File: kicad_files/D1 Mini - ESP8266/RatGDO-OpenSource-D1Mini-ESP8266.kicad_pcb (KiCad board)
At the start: 2 copper layers, 51.8 x 65.8 mm, 24 parts, among them J1 Screw_Terminal_01x03, J2 Conn_01x11, J3 Screw_Terminal_01x02, Q1 2N7002, Q2 AO3400A, Q3 AO3400A, Q4 AO3400A, U1 WeMos_D1_mini, U2 K7805-500R3

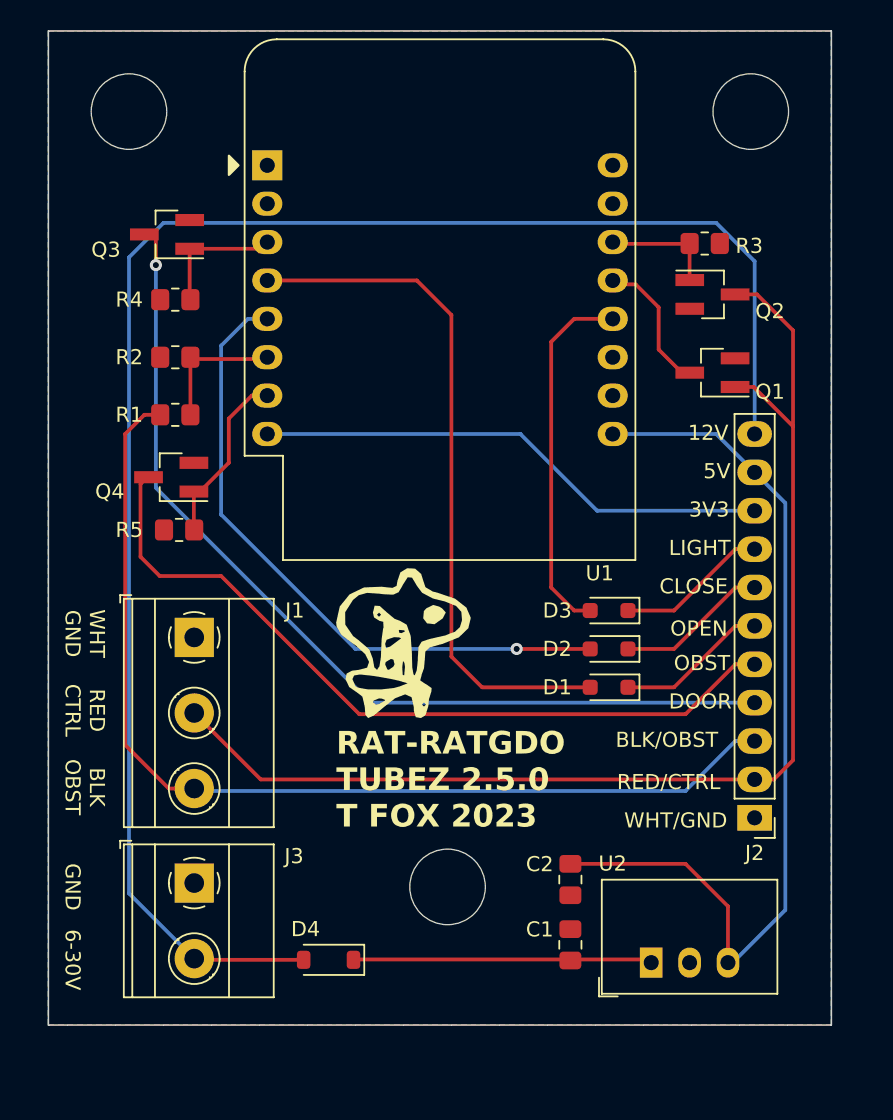
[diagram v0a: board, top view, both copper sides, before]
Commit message: rename
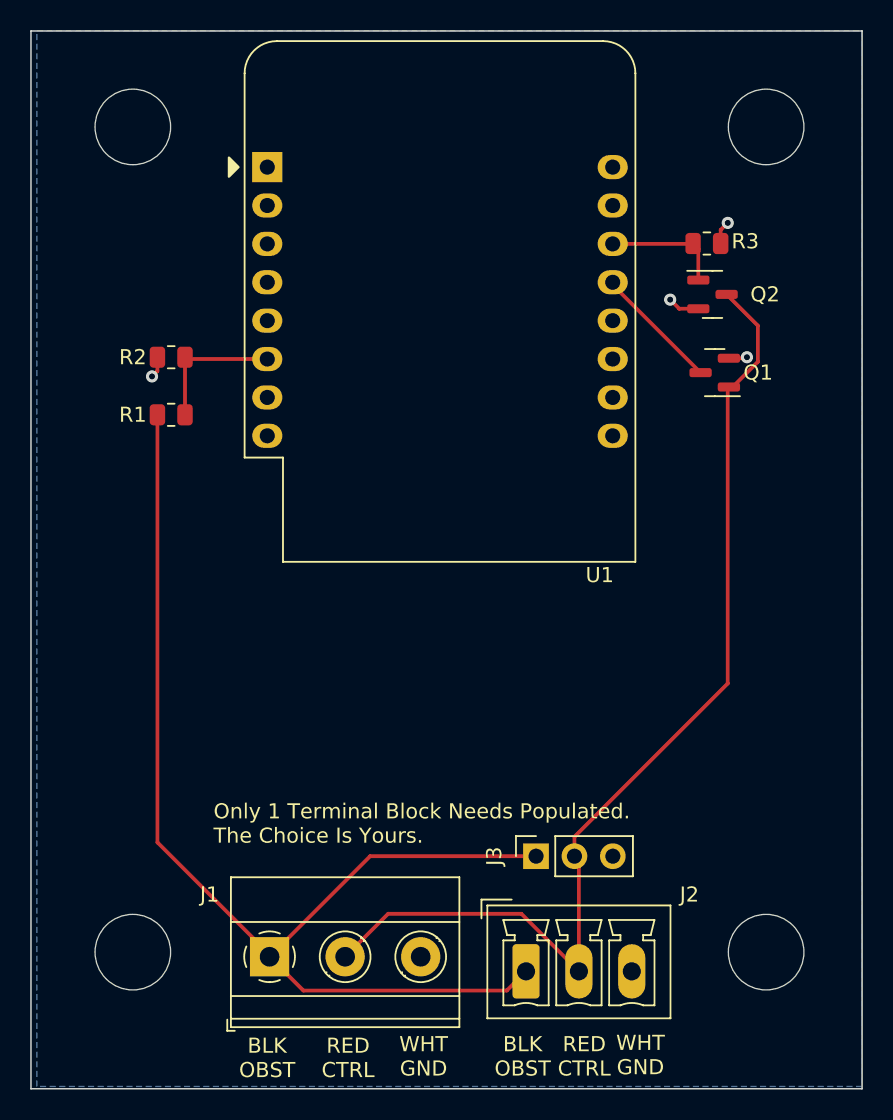
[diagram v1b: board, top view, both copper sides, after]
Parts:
- removed C1: 10uF/50V, Capacitor_SMD:C_0805_2012Metric_Pad1.18x1.45mm_HandSolder
- removed C2: 22uF/10V, Capacitor_SMD:C_0805_2012Metric_Pad1.18x1.45mm_HandSolder
- removed D1, D2, D3: 1N4148WS, Diode_SMD:D_SOD-323_HandSoldering
- removed D4: B5819W, Diode_SMD:D_SOD-123
- removed G***: LOGO, LOGO
- removed Q3, Q4: AO3400A, Package_TO_SOT_SMD:SOT-23_Handsoldering
- removed R4, R5: 10k, Resistor_SMD:R_0805_2012Metric_Pad1.20x1.40mm_HandSolder
- removed U2: K7805-500R3, Converter_DCDC:Converter_DCDC_RECOM_R-78HB-0.5_THT
- added REF**: MountingHole_5mm, MountingHole:MountingHole_5mm, F.Cu at (120.7, 118.1)
- J2: value Conn_01x11 -> Screw_Terminal_01x03; footprint Connector_PinHeader_2.54mm:PinHeader_1x11_P2.54mm_Vertical -> Connector_Phoenix_MC:PhoenixContact_MCV_1,5_3-G-3.5_1x03_P3.50mm_Vertical
- J3: value Screw_Terminal_01x02 -> Screw_Terminal_01x03; footprint TerminalBlock_Phoenix:TerminalBlock_Phoenix_MKDS-1,5-2_1x02_P5.00mm_Horizontal -> Connector_PinSocket_2.54mm:PinSocket_1x03_P2.54mm_Vertical
- Q1, Q2: footprint Package_TO_SOT_SMD:SOT-23_Handsoldering -> Package_TO_SOT_SMD:SOT-23
- R1, R2, R3: footprint Resistor_SMD:R_0805_2012Metric_Pad1.20x1.40mm_HandSolder -> Resistor_SMD:R_0805_2012Metric
- moved J3 22.7 mm to (147.3, 111.8), turned to 90 degrees
- moved J1 21.7 mm to (129.7, 118.4), turned to 0 degrees
- moved REF** 21.5 mm to (162.6, 118.1)
- moved J2 18.2 mm to (146.7, 119.4), turned to 0 degrees
- moved REF** 1.44 mm to (162.6, 63.5)
- moved REF** 1.05 mm to (120.7, 63.5)
- moved R1 0.27 mm to (123.2, 82.5)
- moved R2 0.27 mm to (123.2, 78.7)
- moved Q1 0.15 mm to (159.2, 79.8)
- moved R3 0.14 mm to (158.6, 71.2), turned to 180 degrees
- moved U1 0.12 mm to (129.5, 66.2)
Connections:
- net /ESP_RX renamed Net-(Q1-D)
- J1 pad 1: GND -> Net-(J1-Blk/Obst)
- J1 pad 2: RED/CTRL -> Net-(J1-Red/Cntrl)
- J1 pad 3: BLK/OBST -> GND
- J2 pad 1: GND -> Net-(J1-Blk/Obst)
- J2 pad 2: RED/CTRL -> Net-(J1-Red/Cntrl)
- J2 pad 3: BLK/OBST -> GND
- J3 pad 1: GND -> Net-(J1-Blk/Obst)
- J3 pad 2: +12V -> Net-(J1-Red/Cntrl)
- Q1 pad 1: RED/CTRL -> Net-(J1-Red/Cntrl)
- Q2 pad 1: /ESP_TX -> Net-(Q2-G)
- Q2 pad 3: RED/CTRL -> Net-(J1-Red/Cntrl)
- R1 pad 1: BLK/OBST -> Net-(J1-Blk/Obst)
- R3 pad 1: /ESP_TX -> GND
- R3 pad 2: GND -> Net-(Q2-G)
- U1 pad 12: Net-(D3-A) -> unconnected-(U1-D3-Pad12)
- U1 pad 14: /ESP_TX -> Net-(Q2-G)
- U1 pad 3: Net-(Q3-G) -> unconnected-(U1-D0-Pad3)
- U1 pad 4: Net-(D1-A) -> unconnected-(U1-SCK/D5-Pad4)
- U1 pad 5: Net-(D2-A) -> unconnected-(U1-MISO/D6-Pad5)
- U1 pad 7: Net-(Q4-G) -> unconnected-(U1-CS/D8-Pad7)
- U1 pad 8: +3V3 -> +3.3V
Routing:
- net +12V: track 109.9 -> 0.00 mm
- net RED/CTRL: track 81.3 -> 0.00 mm
- net Net-(J1-Blk/Obst): track 0.00 -> 77.8 mm
- net Net-(J1-Red/Cntrl): track 0.00 -> 69.3 mm
- net BLK/OBST: track 65.7 -> 0.00 mm
- net STS_DOOR: track 62.0 -> 0.00 mm, vias 1 -> 0
- net +5V: track 60.7 -> 0.00 mm
- net STS_OBST: track 51.8 -> 0.00 mm
- net Net-(D1-A): track 45.8 -> 0.00 mm
- net Net-(D2-A): track 43.1 -> 0.00 mm, vias 1 -> 0
- net +3V3: track 34.4 -> 0.00 mm
- net Net-(D3-A): track 24.2 -> 0.00 mm
- net Net-(D4-K): track 19.7 -> 0.00 mm
- net Net-(Q4-G): track 11.3 -> 0.00 mm
- net DC_OPEN: track 10.1 -> 0.00 mm
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- removed copper zone on F.Cu, net GND
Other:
- board size 51.8 x 65.8 mm -> 55 x 70 mm
- board text added: "5v"
- board text added: "EN"
- board text added: "GPIO0"
- board text added: "GPIO1"
- board text added: "GPIO12"
- board text added: "GPIO13"
- board text added: "GPIO14"
- board text added: "GPIO15"
- board text added: "GPIO16"
- board text added: "GPIO2"
- board text added: "GPIO3"
- board text added: "GPIO4"
- board text added: "GPIO5"
- board text added: "Only 1 Terminal Block Needs Populated. The Choice Is Yours."
- board text added: "VCC-3v3"
- board text removed: "12V"
- board text removed: "3V3"
- board text removed: "5V"
- board text removed: "6-30V"
- board text removed: "A0"
- board text removed: "BLK/OBST"
- board text removed: "CLOSE"
- board text removed: "D0"
- board text removed: "D1/SCL"
- board text removed: "D2/SDA"
- board text removed: "D3"
- board text removed: "D4"
- board text removed: "D5/SCK"
- board text removed: "D6/MISO"
- board text removed: "D7/MOSI"
- board text removed: "D8"
- board text removed: "DOOR"
- board text removed: "JLCJLCJLCJLC"
- board text removed: "LIGHT"
- board text removed: "OBST"
- board text removed: "OPEN"
- board text removed: "RAT-RATGDO TUBEZ 2.5.0 T FOX 2023"
- board text removed: "RED/CTRL"
- board text removed: "RX"
- board text removed: "TX"
- board text removed: "WHT/GND"
